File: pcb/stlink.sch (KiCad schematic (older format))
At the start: 41 parts, among them J1 USB_A, Q1 S9013, U1 XC6206P332MR, U2 GD32F103CBT6, Y1 8MHz

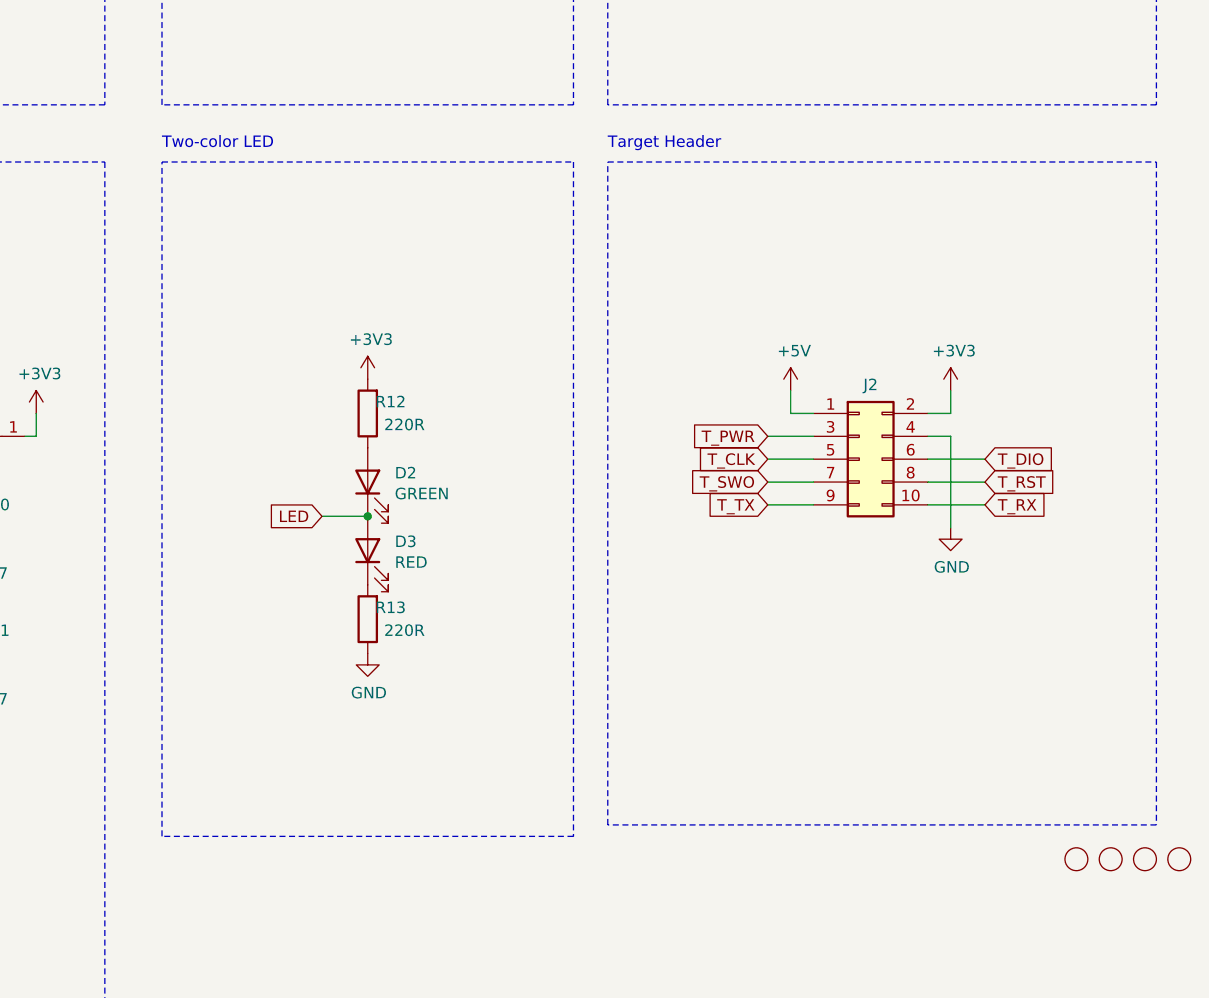
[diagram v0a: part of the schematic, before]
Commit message: Hmmm
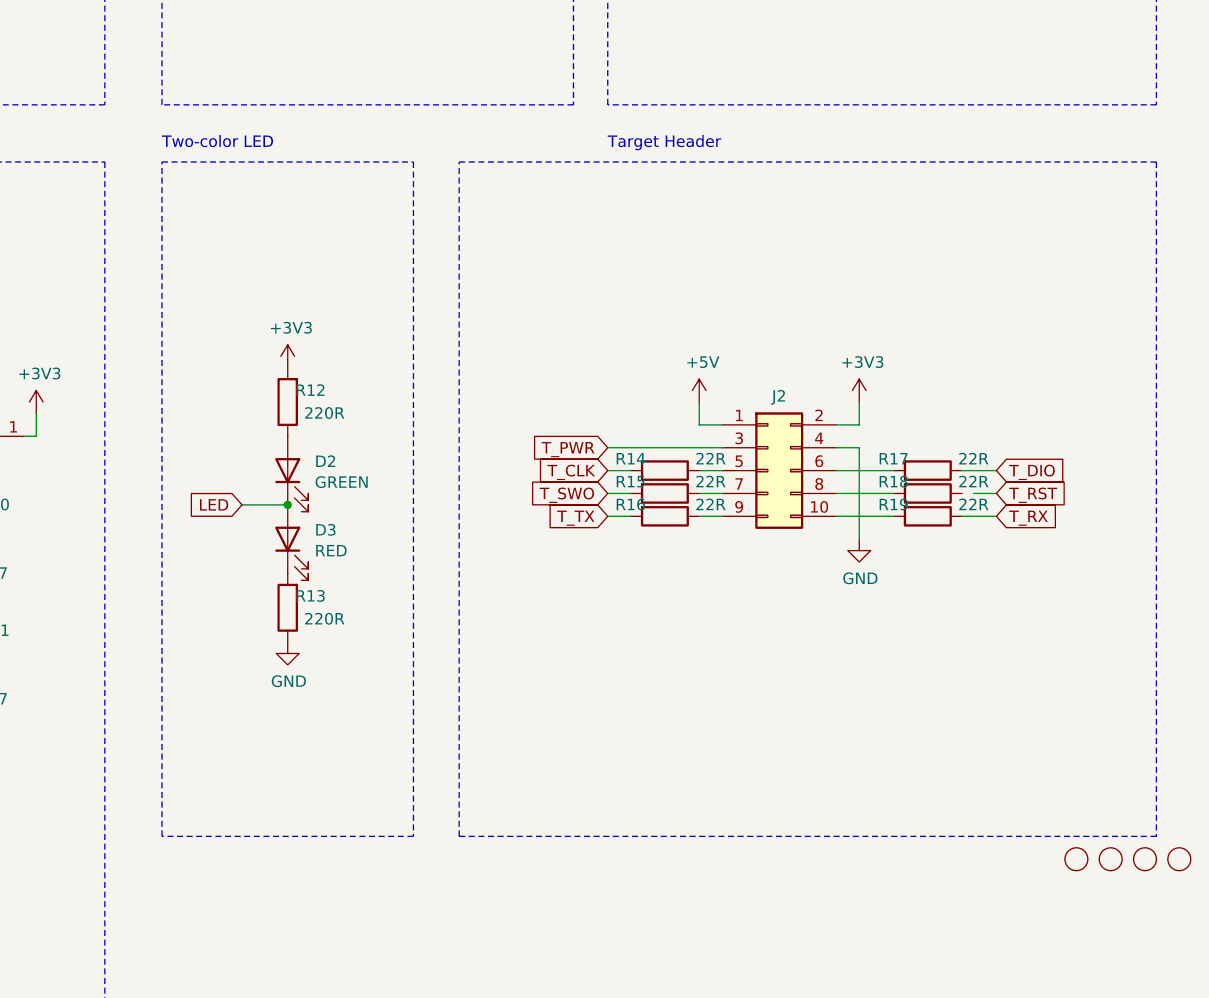
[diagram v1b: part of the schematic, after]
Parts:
- added R14, R15, R16, R17, R18, R19: 22R, Resistor_SMD:R_0402_1005Metric, symbol Device:R
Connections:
- net T_CLK: now also R14.2; no longer J2.5 (Pin_5)
- net T_DIO: now also R17.1; no longer J2.6 (Pin_6)
- net T_RST: no longer J2.8 (Pin_8)
- net T_RX: now also R19.1; no longer J2.10 (Pin_10)
- net T_SWO: now also R15.2; no longer J2.7 (Pin_7)
- net T_TX: now also R16.2; no longer J2.9 (Pin_9)
- new net: J2.10 (Pin_10), R19.2
- new net: J2.5 (Pin_5), R14.1
- new net: J2.6 (Pin_6), R17.2
- new net: J2.7 (Pin_7), R15.1
- new net: J2.8 (Pin_8), R18.2
- new net: J2.9 (Pin_9), R16.1
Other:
- moved on the sheet: D2, D3, J2, R12, R13
